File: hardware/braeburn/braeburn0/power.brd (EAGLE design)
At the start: 100 x 80 mm, 46 parts, among them IC1 7812TV, IC2 7805TV, IC3 7805TV, IC4 ATMEGA48/88/168-AU, IC6 MAX481CSA

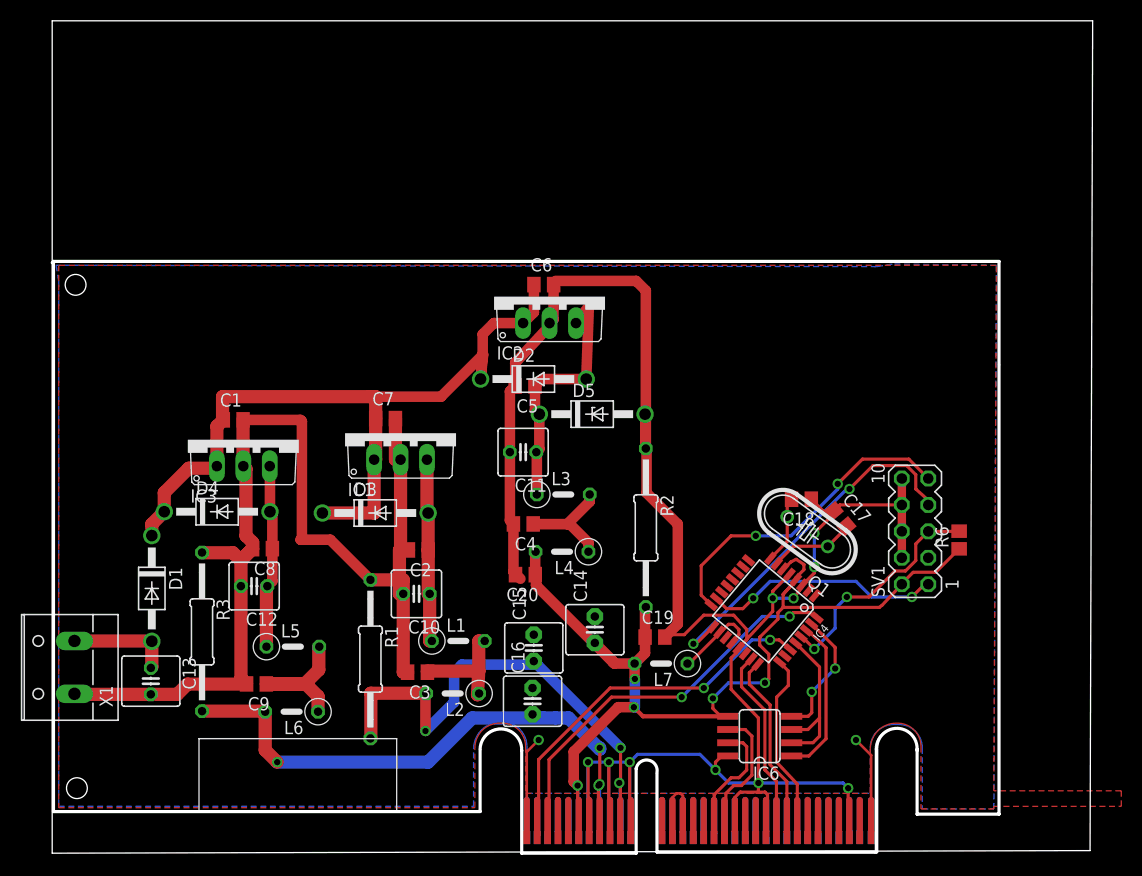
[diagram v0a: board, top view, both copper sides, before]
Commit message: current status
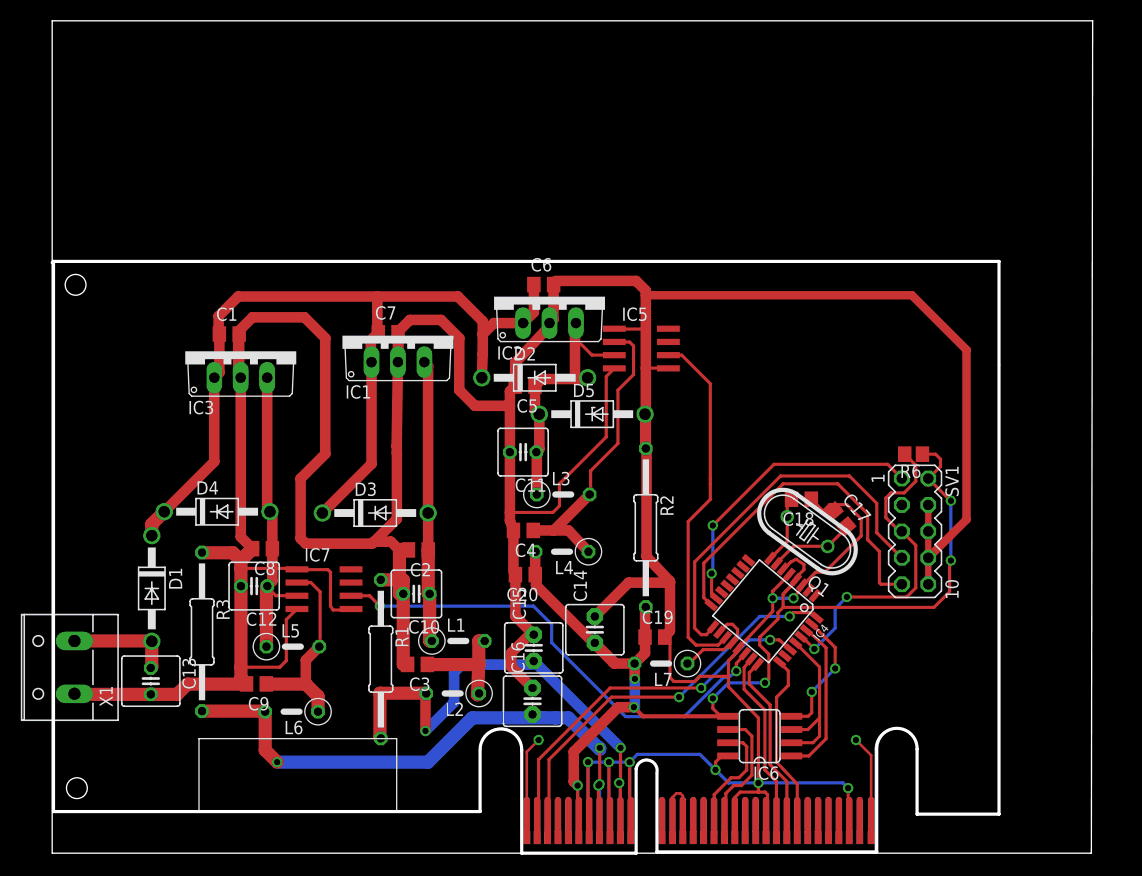
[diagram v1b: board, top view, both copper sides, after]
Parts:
- added IC5, IC7: LM741D, linear:SO08
- moved IC1 9.38 mm to (33.2, 49.7)
- moved R6 9.34 mm to (82.8, 38.4), turned to 180 degrees
- moved IC3 8.50 mm to (18.1, 48.2)
- moved C1 8.26 mm to (17.0, 49.9)
- moved C7 8.25 mm to (32.3, 50.0)
- moved R1 1.00 mm to (31.6, 18.6)
- moved C3 0.75 mm to (35.1, 18.1)
- moved C4 0.62 mm to (45.3, 31.0)
- moved D2 0.18 mm to (46.4, 45.7)
- turned SV1 to 270 degrees
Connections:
- new net 3V3A: C11.1, C5.1, D2.A, D5.C, IC2.3, IC5.3, L3.1
- new net 3V3B: C4.1, IC5.2, L3.2, L4.1
- new net 3V3METER: IC4.19, IC5.6
- new net 5VA: C12.1, C8.1, D4.A, IC3.3, IC7.3, L5.1
- new net 5VB: C9.1, IC7.2, L5.2, L6.1
- new net 5VMETER: IC4.22, IC7.6
- net GND: now also IC5.1, IC5.4, IC5.5, IC7.1, IC7.4, IC7.5, U$1.A27(GND)
- net N$3: now also IC7.7; no longer C12.1, C8.1, D4.A, IC3.3, L5.1
- net N$4: now also IC7.8; no longer C11.1, C5.1, D2.A, D5.C, IC2.3, L3.1
- net N$6: now also IC5.7; no longer C9.1, L5.2, L6.1
- net N$7: now also IC5.8; no longer C4.1, L3.2, L4.1
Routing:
- net GND: track 338.8 -> 519.7 mm, vias 10 -> 8
- net 5VMETER: track 0.00 -> 46.6 mm, vias 0 -> 2
- net 3V3METER: track 0.00 -> 34.6 mm
- net 5VA: track 0.00 -> 29.6 mm
- net 3V3B: track 0.00 -> 28.9 mm
- net 3V3A: track 0.00 -> 26.2 mm
- net N$4: track 25.0 -> 0.00 mm
- net 5VB: track 0.00 -> 19.0 mm
- net N$3: track 17.7 -> 0.00 mm
- net N$6: track 14.8 -> 0.00 mm
- net +3V3: track 104.9 -> 118.9 mm, vias 5 -> 7
- net N$1: track 76.5 -> 88.2 mm
- net N$7: track 10.7 -> 0.00 mm
- net N$5: track 17.9 -> 27.4 mm
- net N$14: track 22.4 -> 31.6 mm
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- removed copper zone on layer 1, net GND
- removed copper zone on layer 16, net GND
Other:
- outline, holes or cut-outs redrawn
